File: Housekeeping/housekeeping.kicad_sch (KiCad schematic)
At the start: 2 parts

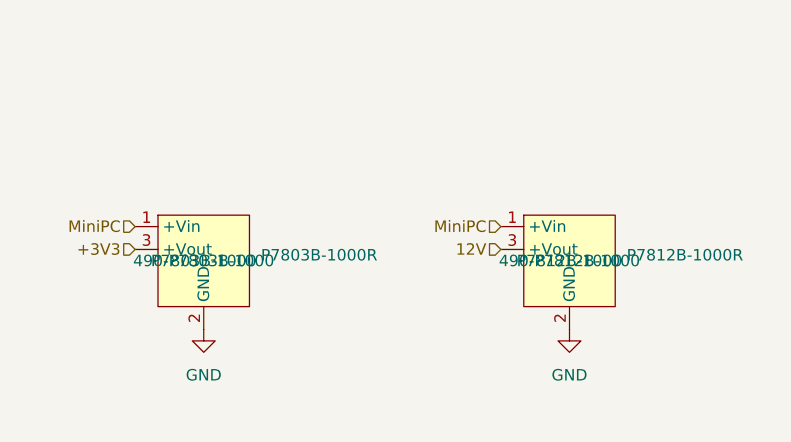
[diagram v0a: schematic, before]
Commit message: began layout
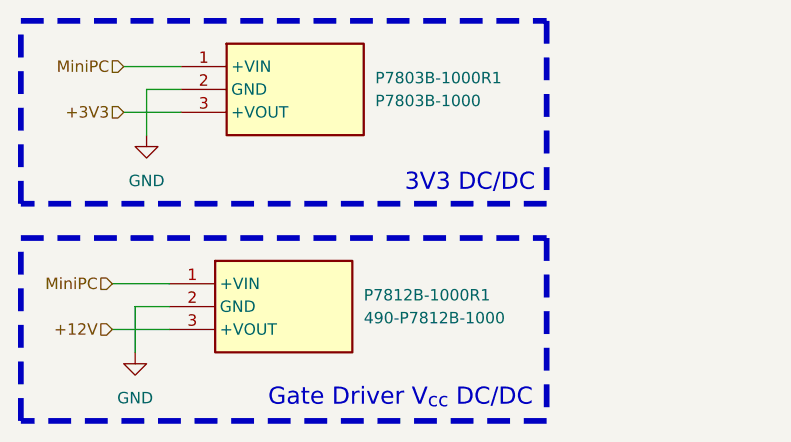
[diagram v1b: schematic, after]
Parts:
- P7803B-1000R1: renamed from P7803B-1000R; value ~ -> P7803B-1000; footprint P78B-1000R series:P78B-1000R -> Robomaster_ICs:P7812B1000; symbol P78B-1000R series:P78B-1000R -> Robomaster_IV:P7803B-1000; Height (none) -> 10.45; Manufacturer_Name (none) -> CUI Inc.; Mouser Price/Stock (none) -> https://www.mouser.com/ProductDetail/CUI-Inc/P7803B-1000?qs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
- P7812B-1000R1: renamed from P7812B-1000R; value ~ -> 490-P7812B-1000; footprint P78B-1000R series:P78B-1000R -> Robomaster_ICs:P7812B1000; symbol P78B-1000R series:P78B-1000R -> Robomaster_IV:P7812B-1000; Height (none) -> 10.45; Manufacturer_Name (none) -> CUI Inc.; Mouser Price/Stock (none) -> https://www.mouser.com/ProductDetail/CUI-Inc/P7812B-1000?qs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
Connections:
- net 12V renamed +12V
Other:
- note added: "3V3 DC/DC"
- note added: "Gate Driver V_{cc} DC/DC"
- moved on the sheet: P7803B-1000R1, P7812B-1000R1
